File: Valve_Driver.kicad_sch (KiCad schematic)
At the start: 5 parts, among them J10 Conn_01x02, J11 Conn_01x02, U1 TC1508S

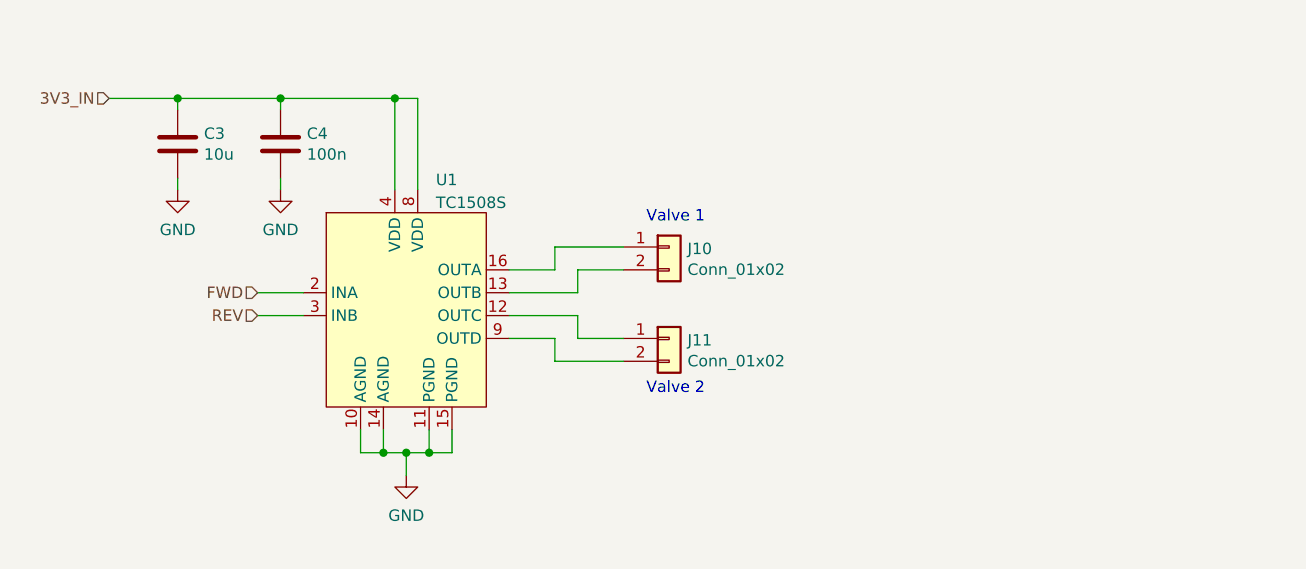
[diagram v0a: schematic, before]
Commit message: Finalize schematic
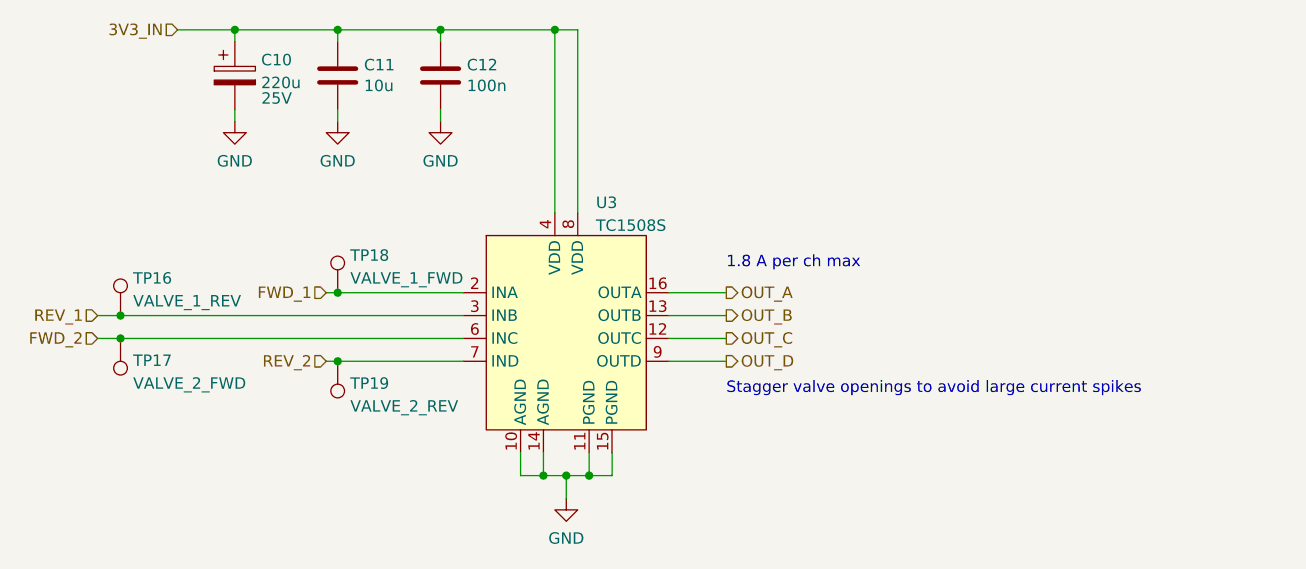
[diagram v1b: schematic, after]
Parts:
- removed J10, J11: Conn_01x02, co2_sensor_node:KF301-5.0-2P, symbol Connector_Generic:Conn_01x02
- added C10: 220u, Capacitor_THT:CP_Radial_D8.0mm_P3.50mm, symbol Device:C_Polarized
- added TP16: VALVE_1_REV, TestPoint:TestPoint_Loop_D2.50mm_Drill1.0mm_LowProfile, symbol Connector:TestPoint
- added TP17: VALVE_2_FWD, TestPoint:TestPoint_Loop_D2.50mm_Drill1.0mm_LowProfile, symbol Connector:TestPoint
- added TP18: VALVE_1_FWD, TestPoint:TestPoint_Loop_D2.50mm_Drill1.0mm_LowProfile, symbol Connector:TestPoint
- added TP19: VALVE_2_REV, TestPoint:TestPoint_Loop_D2.50mm_Drill1.0mm_LowProfile, symbol Connector:TestPoint
- renumbered C3 to C11, C4 to C12, U1 to U3
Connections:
- net 3V3_IN: now also C10.1
- net GND: now also C10.2
- net OUT_C: now reaches U3.12 (OUTC)
- net OUT_B: now reaches U3.13 (OUTB)
- net OUT_A: now reaches U3.16 (OUTA)
- net OUT_D: now reaches U3.9 (OUTD)
- net FWD renamed FWD_1
- net FWD_1: now also TP18.1
- net REV renamed REV_1
- net REV_1: now also TP16.1
- new net FWD_2: TP17.1, U3.6 (INC)
- new net REV_2: TP19.1, U3.7 (IND)
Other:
- note added: "1.8 A per ch max"
- note added: "Stagger valve openings to avoid large current spikes"
- note removed: "Valve 1"
- note removed: "Valve 2"
- title: (none) -> CO2 Chamber - Valve Driver
- moved on the sheet: C11, C12
